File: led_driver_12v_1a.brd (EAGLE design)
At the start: 45 x 19.4 mm, 53 parts, among them Q1 BSZ0902NSI, Q2 BSZ0902NSI, Q3 BSZ0902NSI, Q4 BSZ0902NSI, Q5 BSZ0902NSI, Q6 SSM3K2615R

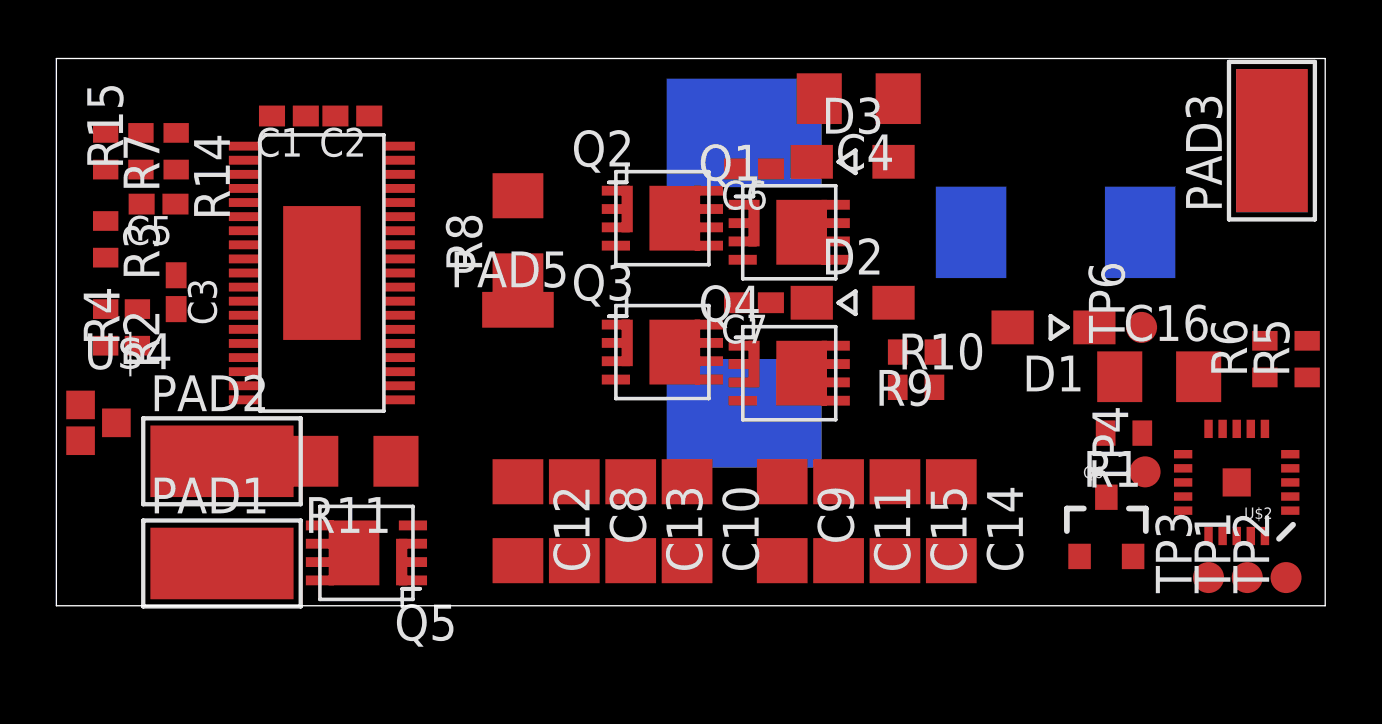
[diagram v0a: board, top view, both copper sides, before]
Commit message: routing complete. main tasks to do: add polys, optimize routes width, add some extra vias, make gerbers
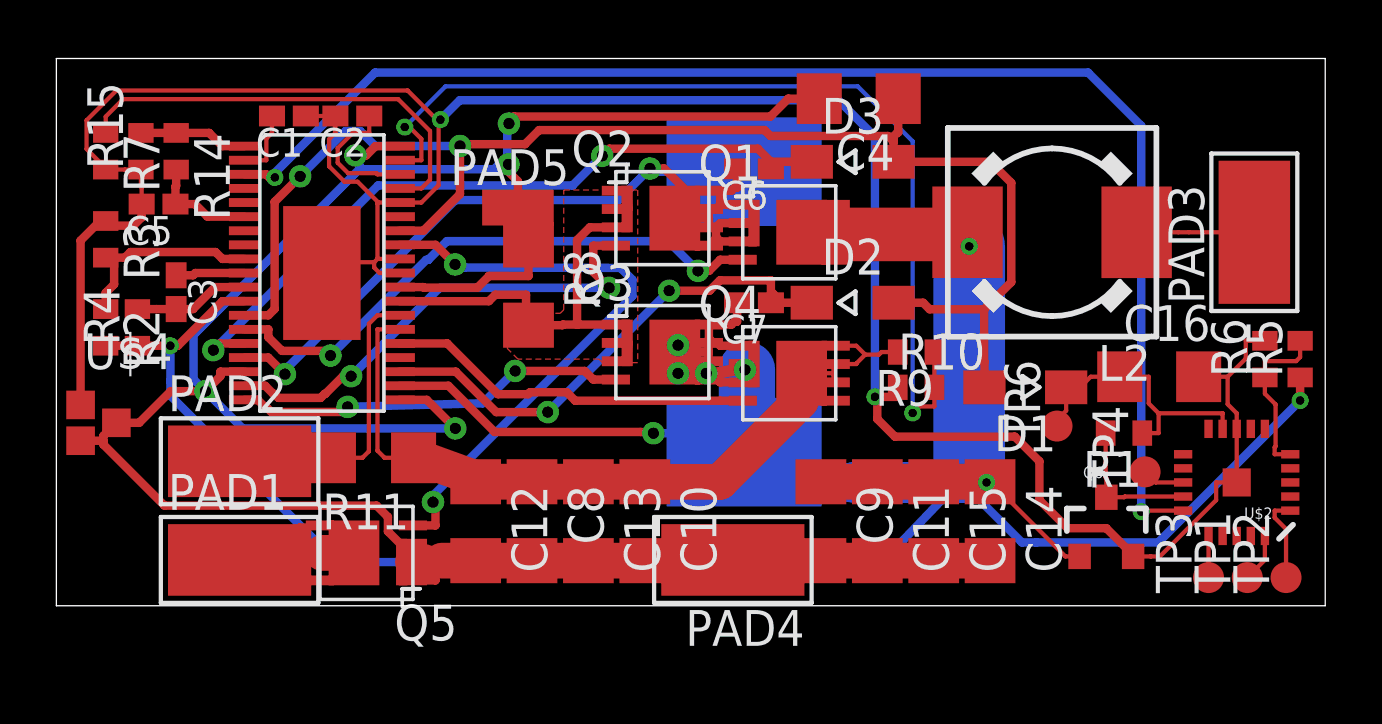
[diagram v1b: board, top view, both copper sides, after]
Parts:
- moved PAD4 24.2 mm to (24.0, 1.62), flipped to the top, turned to 90 degrees
- moved TP6 4.61 mm to (35.5, 6.38)
- moved PAD5 3.62 mm to (16.4, 14.1)
- moved PAD3 3.31 mm to (42.5, 13.2)
- moved D1 2.35 mm to (34.4, 7.75)
- moved R8 1.79 mm to (16.8, 11.4), turned to 270 degrees
- moved C10 1.50 mm to (20.9, 3.00)
- moved C12 1.50 mm to (14.9, 3.00)
- moved C13 1.50 mm to (18.9, 3.00)
- moved C8 1.50 mm to (16.9, 3.00)
- moved C11 1.38 mm to (29.1, 3.00)
- moved C14 1.38 mm to (33.1, 3.00)
- moved C15 1.38 mm to (31.1, 3.00)
- moved C9 1.38 mm to (27.1, 3.00)
- moved L1 1.38 mm to (24.4, 10.4)
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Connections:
- removed net N$10: C7.2, L1.2, Q3.D, Q3.D@1, Q3.D@2, Q3.D@3, Q3.D@4, Q4.S@1, Q4.S@2, Q4.S@3, Q4.S@4
- removed net N$8: C6.2, L1.1, Q1.S@1, Q1.S@2, Q1.S@3, Q1.S@4, Q2.D, Q2.D@1, Q2.D@2, Q2.D@3, Q2.D@4
- net SNSN: now also R8.1; no longer R8.2
- net SNSP: now also R8.2; no longer R8.1
- net SW1: now also C6.2, L1.1, Q1.S@1, Q1.S@2, Q1.S@3, Q1.S@4, Q2.D, Q2.D@1, Q2.D@2, Q2.D@3, Q2.D@4
- net SW2: now also C7.2, L1.2, Q3.D, Q3.D@1, Q3.D@2, Q3.D@3, Q3.D@4, Q4.S@1, Q4.S@2, Q4.S@3, Q4.S@4
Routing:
- net +12V: track 0.00 -> 104.3 mm, vias 0 -> 4
- net DGND: track 0.00 -> 95.2 mm, vias 0 -> 2
- net GND: track 0.00 -> 90.8 mm, vias 0 -> 5
- net INTVCC: track 0.00 -> 50.8 mm, vias 0 -> 2
- net N$14: track 0.00 -> 49.6 mm, vias 0 -> 2
- net N$6: track 0.00 -> 34.2 mm, vias 0 -> 2
- net SW1: track 0.00 -> 32.4 mm, vias 0 -> 2
- net ISP: track 0.00 -> 31.2 mm
- net SW2: track 0.00 -> 29.5 mm, vias 0 -> 5
- net BST1: track 0.00 -> 25.8 mm, vias 0 -> 2
- net PWMOUT: track 0.00 -> 21.3 mm, vias 0 -> 2
- net TG1: track 0.00 -> 20.5 mm, vias 0 -> 2
- net SNSP: track 0.00 -> 18.5 mm
- net BST2: track 0.00 -> 18.1 mm, vias 0 -> 2
- net BG1: track 0.00 -> 17.3 mm, vias 0 -> 2
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- added copper zone on layer 1, net SNSP
